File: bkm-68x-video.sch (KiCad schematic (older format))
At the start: 71 parts, among them J1 PR_R, J10 TP_VIDEO_OE, J11 TP_VSYNC, J13 PR_R_OUT, J15 Y_G_OUT, J16 PB_B_OUT, J17 EXT_SYNC_OUT, J2 Y_G, J3 PB_B, J4 EXT_SYNC, J5 TP_Y_G, J6 TP_PB_B, J7 TP_PR_R, J8 TP_HSYNC, J9 TP_INT_EXT_SYNC, Q1 MMBT3904, SW3 PR_R_TERM, SW4 Y_G_TERM, SW5 PB_B_TERM, SW6 EXT_SYNC_TERM, U1 ADG1611BCPZ, U16 SN74LVC1G14DBV, U17 ISL4089, U2 THS7374, U3 ISL59885, U4 ADG734, U8 TC7WH125

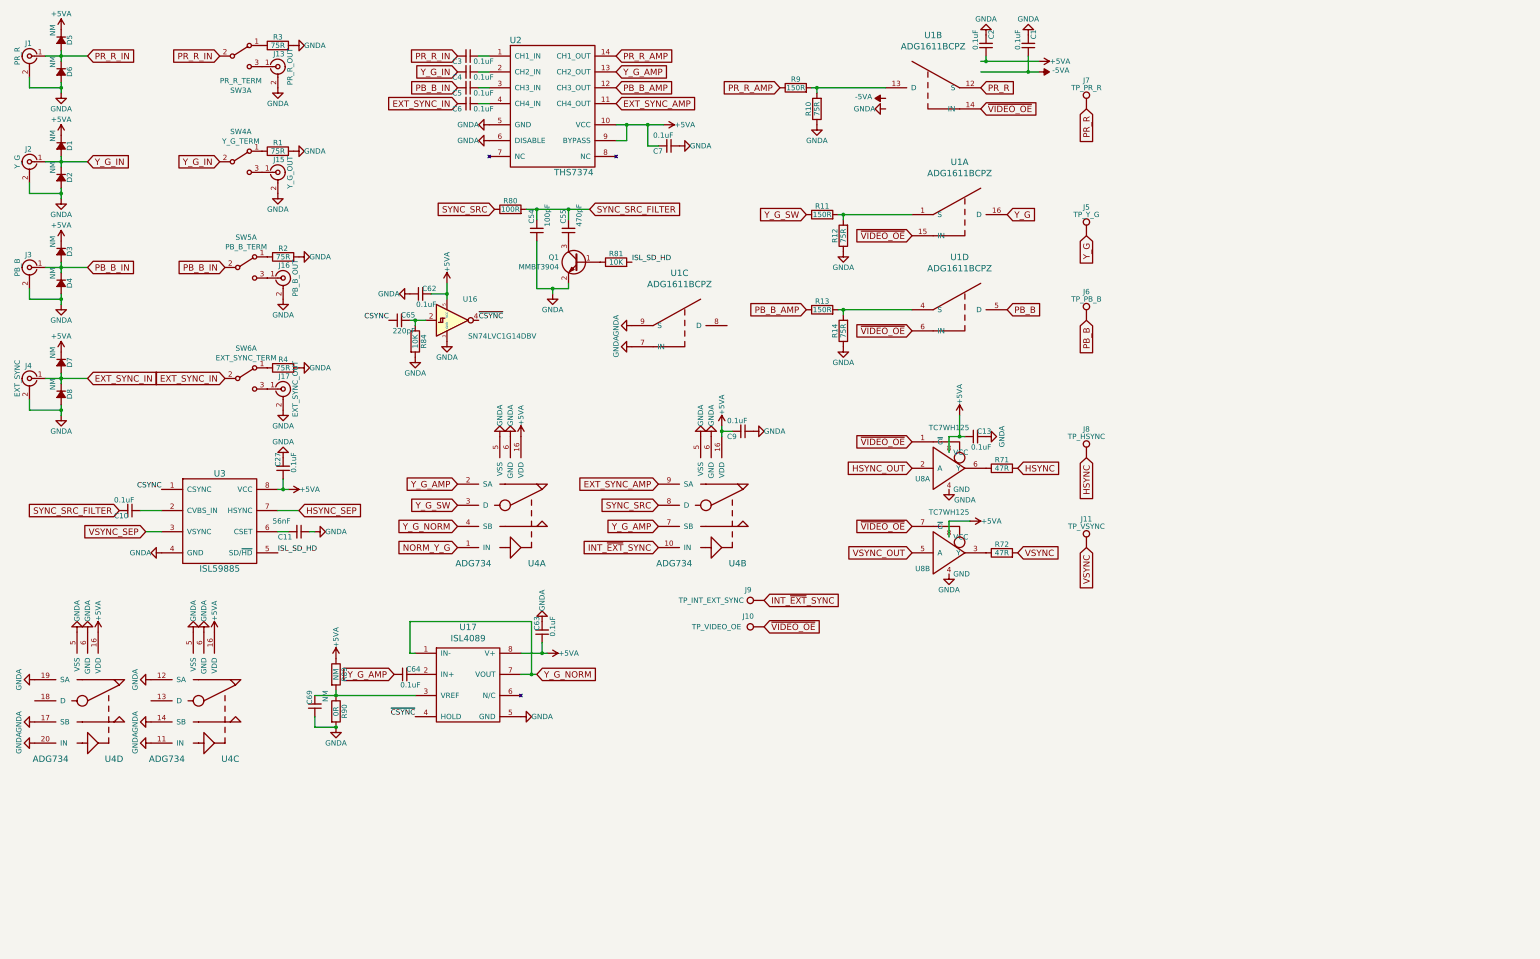
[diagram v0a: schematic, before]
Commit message: Rev. F1
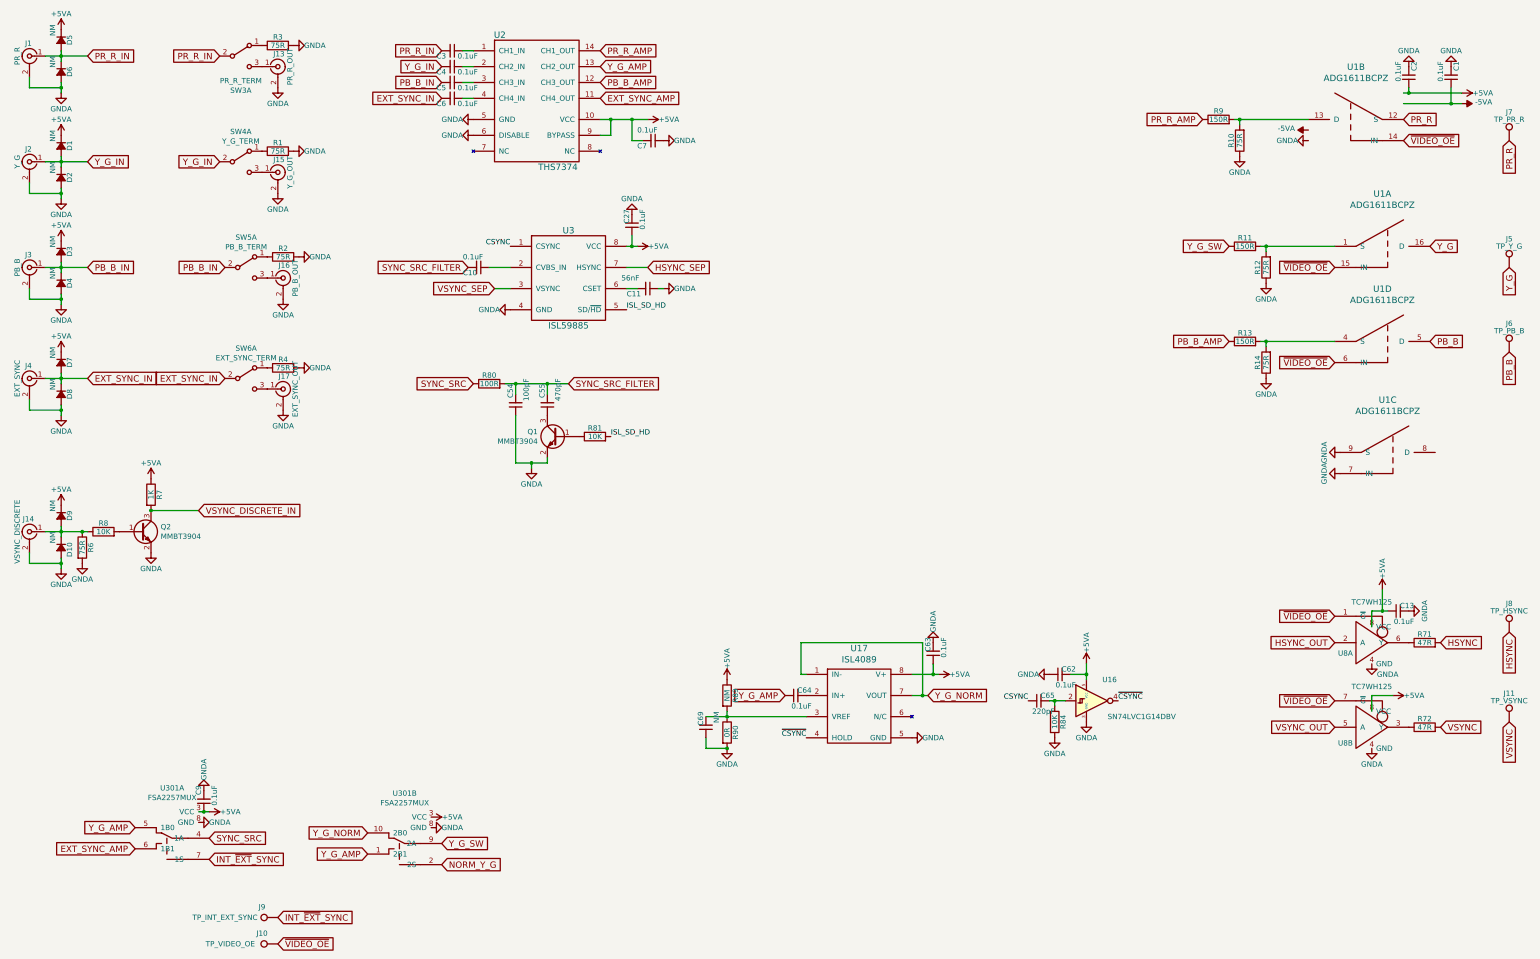
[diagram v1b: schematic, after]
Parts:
- removed U4: ADG734, Package_SO:TSSOP-20_4.4x6.5mm_P0.65mm, symbol adg734:ADG734
- added D10, D9: NM, Diode_SMD:D_SOD-123, symbol bkm-68x-simple-rescue:D_Small_ALT
- added J14: VSYNC_DISCRETE, BNC-THT:BNC-THT, symbol bkm-68x-simple-rescue:Conn_Coaxial
- added Q2: MMBT3904, Package_TO_SOT_SMD:SOT-23_Handsoldering, symbol Device:Q_NPN_BEC
- added R6: 75R, Resistor_SMD:R_0805_2012Metric_Pad1.20x1.40mm_HandSolder, symbol bkm-68x-simple-rescue:R
- added R7: 1K, Resistor_SMD:R_0805_2012Metric_Pad1.20x1.40mm_HandSolder, symbol bkm-68x-simple-rescue:R
- added R8: 10K, Resistor_SMD:R_0805_2012Metric_Pad1.20x1.40mm_HandSolder, symbol bkm-68x-simple-rescue:R
- added U301: FSA2257MUX, Package_SO:MSOP-10_3x3mm_P0.5mm, symbol FSA2257:FSA2257MUX
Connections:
- net +5VA: now also C9.1, D9.1 (K), R7.1, U301.3 (VCC), U301.3 (VCC); no longer C9.2
- net EXT_SYNC_AMP: now also U301.6 (1B1)
- net GND: now also C9.2, D10.2 (A), J14.2 (Ext), Q2.2 (E), R6.2, U301.8 (GND), U301.8 (GND); no longer C9.1
- net INT_~EXT~_SYNC: now also U301.7 (1S)
- net NORM_Y_G: now also U301.2 (2S)
- net SYNC_SRC: now also U301.4 (1A)
- net Y_G_AMP: now also U301.1 (2B1), U301.5 (1B0)
- net Y_G_NORM: now also U301.10 (2B0)
- net Y_G_SW: now also U301.9 (2A)
- new net: D10.1 (K), D9.2 (A), J14.1 (In), R6.1, R8.1
- new net: Q2.1 (B), R8.2
- new net VSYNC_DISCRETE_IN: Q2.3 (C), R7.2
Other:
- moved on the sheet: C1, C10, C11, C13, C2, C27, C3, C4, C5, C54, C55, C6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
